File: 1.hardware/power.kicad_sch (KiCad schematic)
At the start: 53 parts, among them IC1 TLE8366E_V33, IC4 TPS7A2018PDBVR, J4 12V~24V BAT, J5 12V-24V Jack, J9 Conn_01x02, Q4 PMOS, U6 LM2931-5.0_SO8

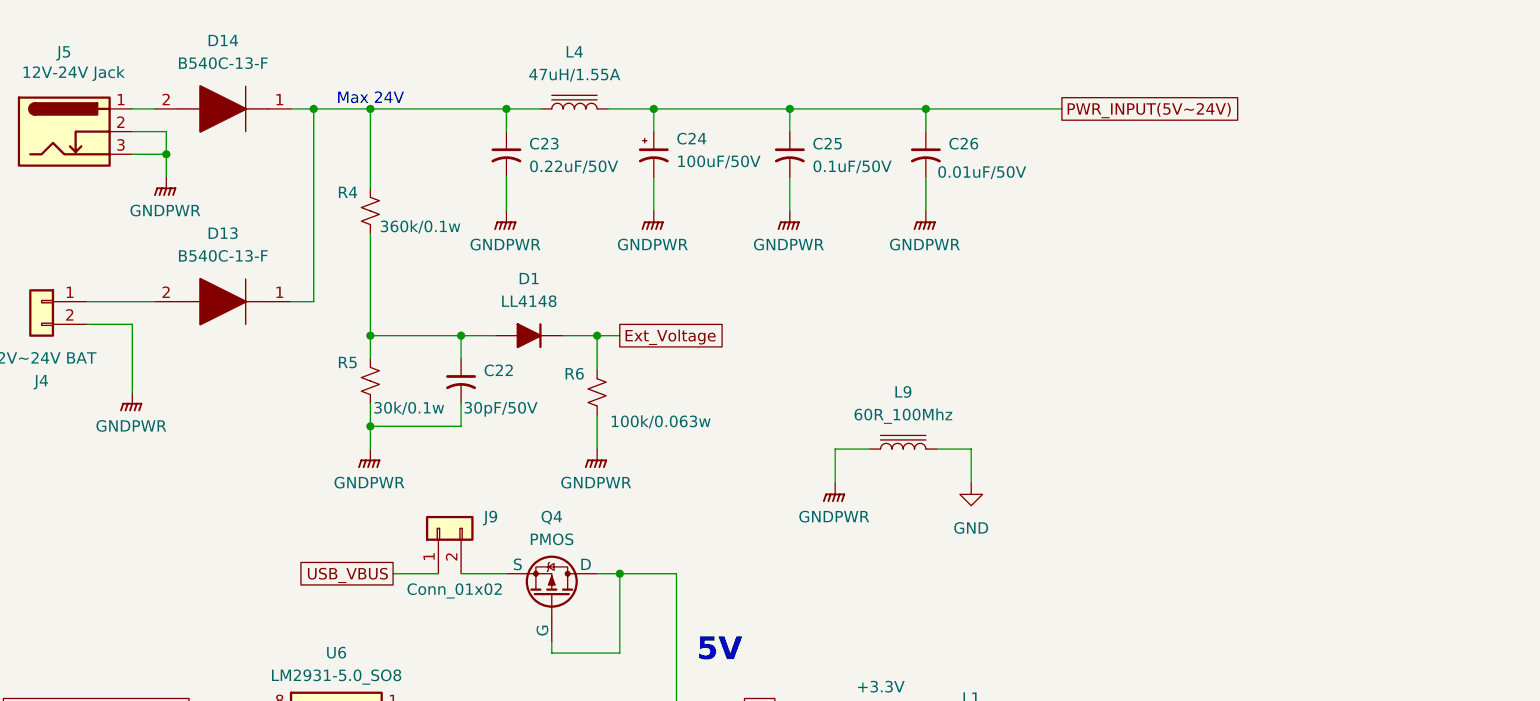
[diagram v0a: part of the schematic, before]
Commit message: 중간저장
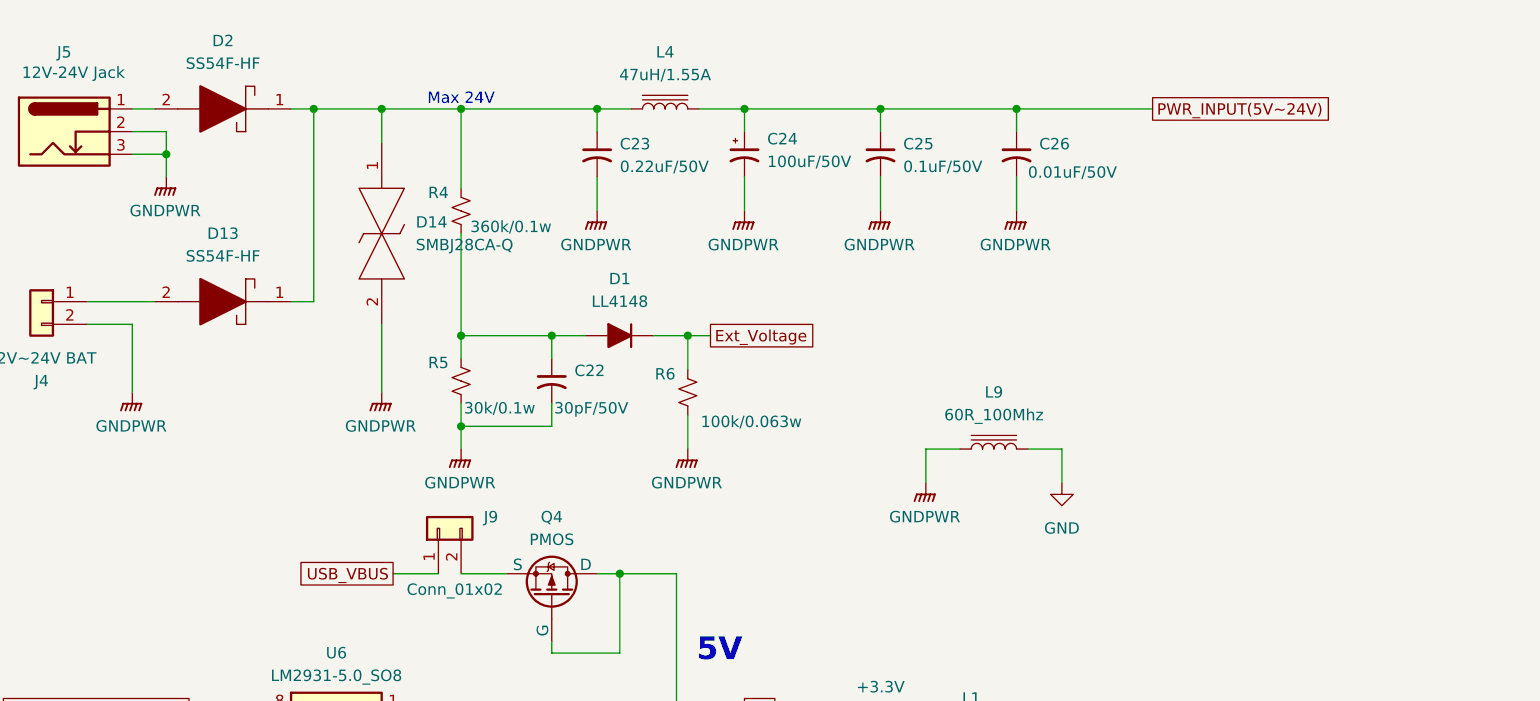
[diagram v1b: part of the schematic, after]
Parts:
- removed D13, D14: B540C-13-F, DIOM7959X250N, symbol SamacSys_Parts:B540C-13-F
- added D13, D2: SS54F-HF, SODFL4626X120N, symbol SamacSys_Parts:SS54F-HF
- added D14: SMBJ28CA-Q, DIONM5436X244N, symbol SamacSys_Parts:SMBJ28CA-Q
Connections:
- net GNDPWR: now also D14.2
- net at C23.1, L4.1, R4.2: now also D13.1, D14.1, D2.1
- net at J5.1: now also D2.2
- net at J4.1 (Pin_1): now also D13.2
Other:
- moved on the sheet: C22, C23, C24, C25, C26, D1, L4, L9, R4, R5, R6

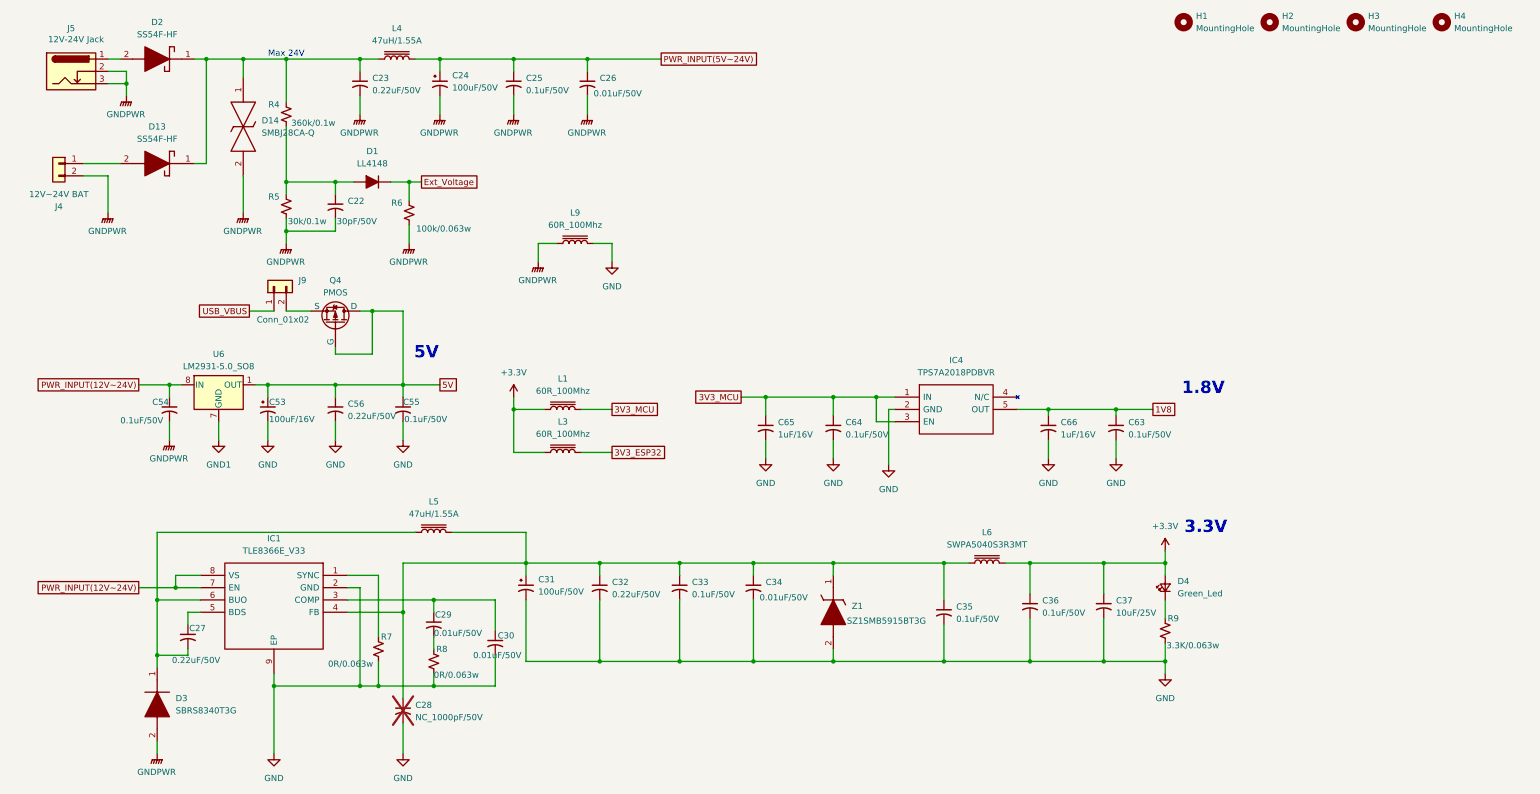
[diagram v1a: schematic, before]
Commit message: 중간 저장
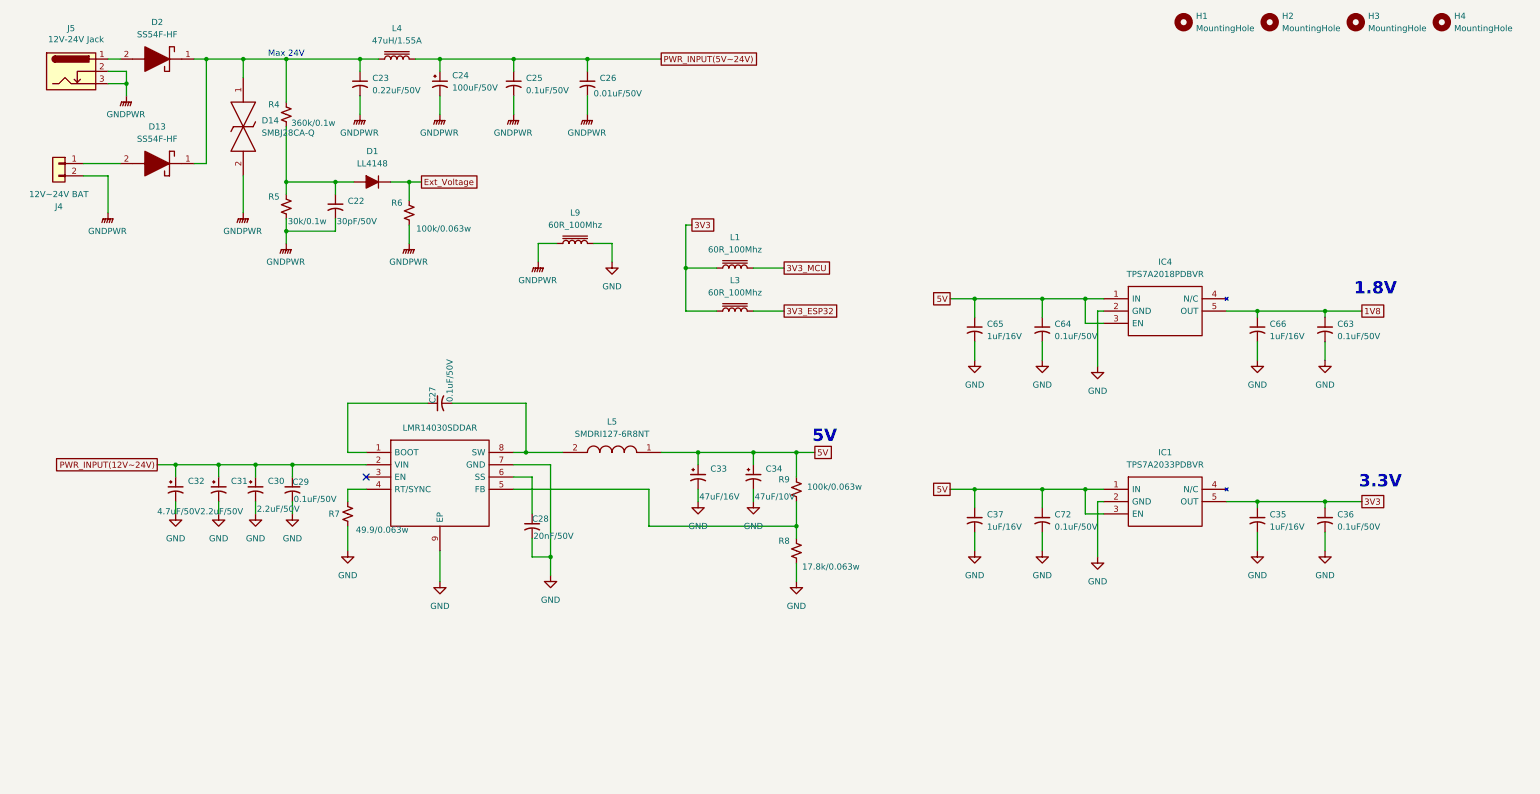
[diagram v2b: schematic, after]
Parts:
- removed C30, C34: 0.01uF/50V, Capacitor_SMD:C_0402_1005Metric, symbol Device:C_Small_US
- removed C32, C56: 0.22uF/50V, Capacitor_SMD:C_0603_1608Metric, symbol Device:C_Small_US
- removed C33, C54, C55: 0.1uF/50V, Capacitor_SMD:C_0402_1005Metric, symbol Device:C_Small_US
- removed C53: 100uF/16V, Capacitor_THT:CP_Radial_Tantal_D8.0mm_P5.00mm, symbol Device:C_Polarized_Small_US
- removed D3: SBRS8340T3G, symbol SamacSys_Parts:SBRS8340T3G
- removed D4: Green_Led, LED_SMD:LED_0603_1608Metric, symbol Device:LED_Small
- removed IC1: TLE8366E_V33, SamacSys_Parts:SOIC127P600X170-9N, symbol SamacSys_Parts:TLE8366E_V50
- removed J9: Conn_01x02, symbol Connector_Generic:Conn_01x02
- removed L5: 47uH/1.55A, Inductor_SMD:L_SXN_SMDRI127, symbol Device:L_Iron
- removed L6: SWPA5040S3R3MT, Inductor_SMD:L_Sunlord_SWPA5040S, symbol Device:L_Iron
- removed Q4: PMOS, symbol Simulation_SPICE:PMOS
- removed U6: LM2931-5.0_SO8, Package_SO:SOIC-8_3.9x4.9mm_P1.27mm, symbol Regulator_Linear:LM2931-5.0_SO8
- removed Z1: SZ1SMB5915BT3G, SamacSys_Parts:DIOM5436X247N, symbol SamacSys_Parts:SZ1SMB5915BT3G
- added C30: 2.2uF/50V, symbol Device:C_Polarized_Small_US
- added C32: 4.7uF/50V, symbol Device:C_Polarized_Small_US
- added C33: 47uF/16V, symbol Device:C_Polarized_Small_US
- added C34: 47uF/10V, symbol Device:C_Polarized_Small_US
- added C72: 0.1uF/50V, Capacitor_SMD:C_0402_1005Metric, symbol Device:C_Small_US
- added IC1: TPS7A2033PDBVR, SOT95P280X145-5N, symbol SamacSys_Parts:TPS7A2033PDBVR
- added IC5: LMR14030SDDAR, SOIC127P600X170-9N, symbol SamacSys_Parts:LMR14030SDDAR
- added L5: SMDRI127-6R8NT, SMDRI1276R8NT, symbol SamacSys_Parts:SMDRI127-6R8NT
- C27: value 0.22uF/50V -> 0.1uF/50V; footprint Capacitor_SMD:C_0603_1608Metric -> Capacitor_SMD:C_0402_1005Metric
- C28: value NC_1000pF/50V -> 20nF/50V; now fitted; now in the parts list
- C29: value 0.01uF/50V -> 0.1uF/50V
- C31: value 100uF/50V -> 2.2uF/50V; footprint Capacitor_THT:CP_Radial_Tantal_D8.0mm_P5.00mm -> (none)
- C35: value 0.1uF/50V -> 1uF/16V
- C37: value 10uF/25V -> 1uF/16V; footprint Capacitor_SMD:C_1206_3216Metric -> Capacitor_SMD:C_0402_1005Metric
- R7: value 0R/0.063w -> 49.9/0.063w; footprint Resistor_SMD:R_0402_1005Metric -> (none)
- R8: value 0R/0.063w -> 17.8k/0.063w; footprint Resistor_SMD:R_0402_1005Metric -> (none)
- R9: value 3.3K/0.063w -> 100k/0.063w; footprint Resistor_SMD:R_0402_1005Metric -> (none)
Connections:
- net 3V3_MCU: no longer C64.1, C65.1, IC4.1 (IN), IC4.3 (EN)
- net 5V: now also C37.1, C64.1, C65.1, IC4.1 (IN), IC4.3 (EN), R9.2, C33.1, C34.1, C72.1, IC1.1 (IN), IC1.3 (EN), L5.1
- net GND: now also C29.2, R7.1, R8.1, C30.2, C32.2, C33.2, C34.2, C72.2, IC1.2 (GND), IC5.7 (GND), IC5.9 (EP); no longer R7.2, R8.2, R9.2
- net PWR_INPUT(12V~24V): now also C29.1, C31.1, C30.1, C32.1, IC5.2 (VIN)
- net at R9.1: now also R8.2, IC5.5 (FB)
- net at C27.2: now also IC5.8 (SW), L5.2
- net at C27.1: now also IC5.1 (BOOT)
- net +3.3V renamed 3V3
- net 3V3: now also C35.1, IC1.5 (OUT); no longer C37.1
- new net: C28.1, IC5.6 (SS)
- new net: IC5.4 (RT/SYNC), R7.2
- no-connect marks 0 -> 1
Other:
- moved on the sheet: C63, C64, C65, C66, IC4, L1, L3
